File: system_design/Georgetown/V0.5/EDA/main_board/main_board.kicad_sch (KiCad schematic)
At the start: 23 parts, among them U1 top_rail_v2, U2 DS3231M, U3 INA219AxD, U5 KA78M05_TO252

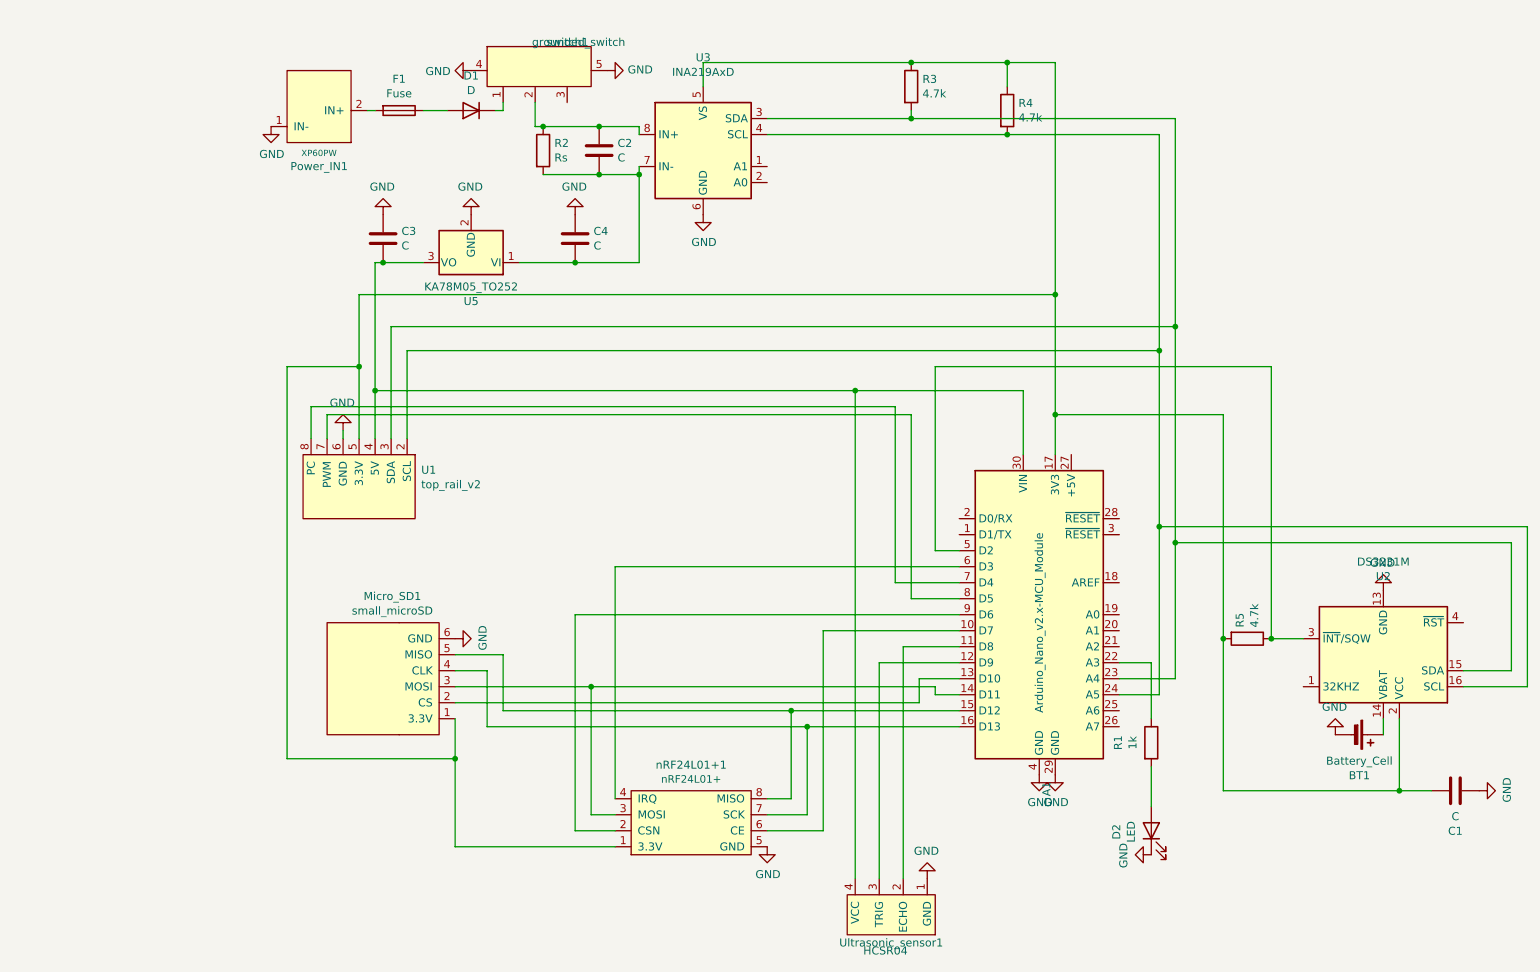
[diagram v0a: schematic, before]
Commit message: PCB modified
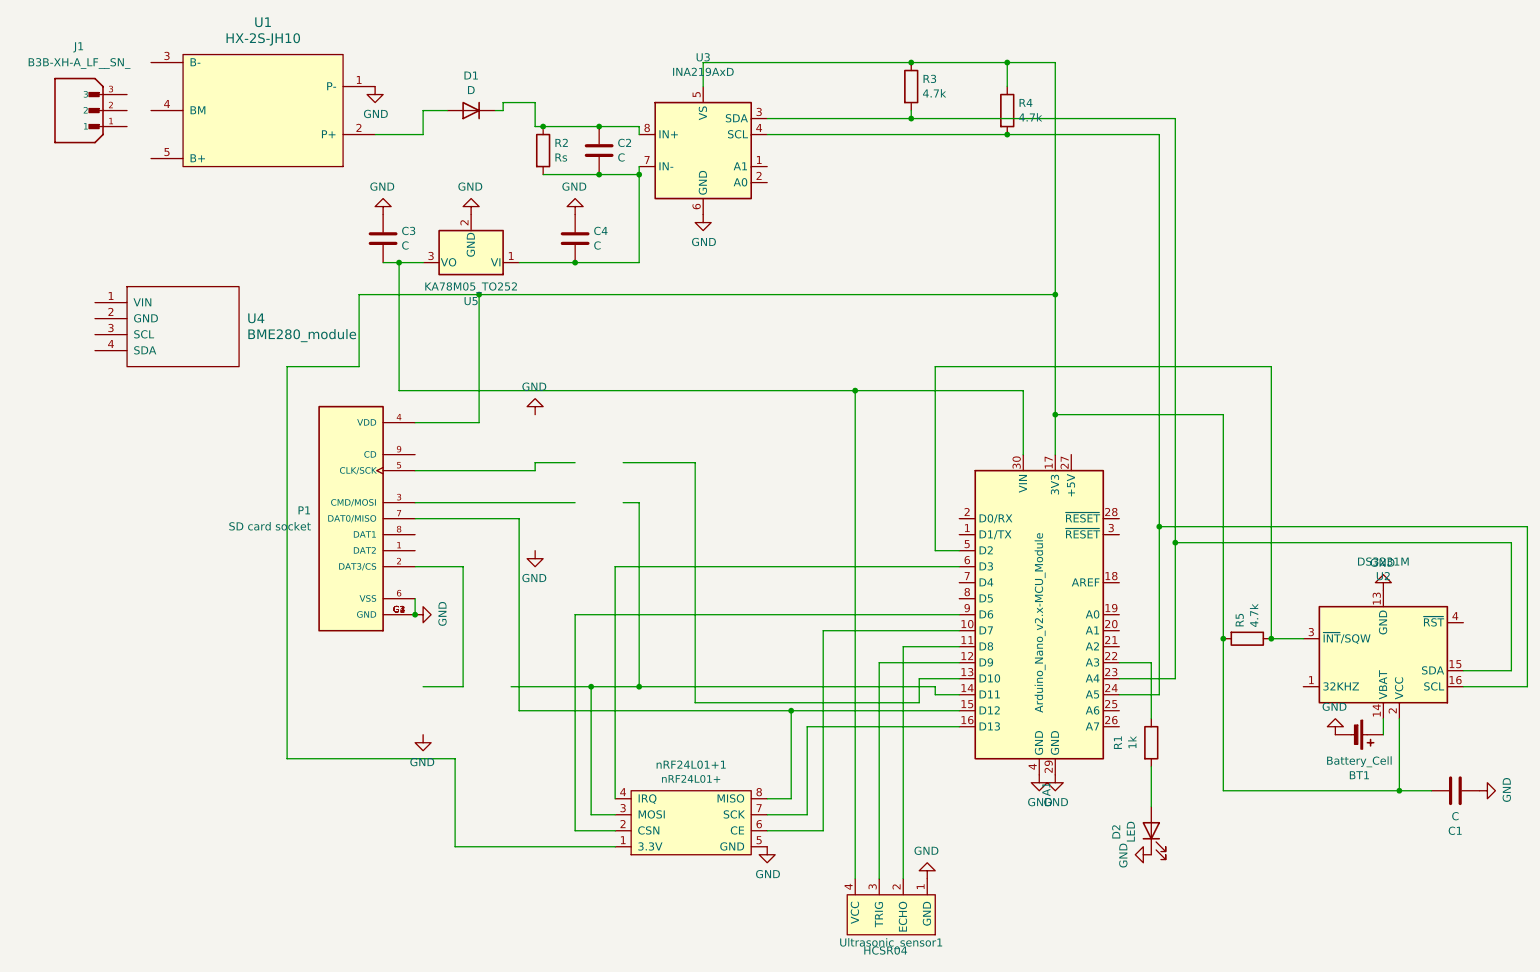
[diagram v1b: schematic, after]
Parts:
- removed F1: Fuse, Resistor_SMD:R_0603_1608Metric_Pad1.05x0.95mm_HandSolder, symbol Device:Fuse
- removed Micro_SD1: small_microSD, ARTS-Lab:small_microSD_v2, symbol main_board-rescue:small_microSD-whs5-rescue
- removed Power_IN1: XP60PW, ARTS-Lab:XT60PW, symbol main_board-rescue:XP60PW-whs5-rescue-whs5-rescue
- removed U1: top_rail_v2, ARTS-Lab:top_rail_v2, symbol main_board-rescue:top_rail_v2-ARTS-Lab
- removed switch1: grounded_switch, ARTS-Lab:grounded_switch, symbol main_board-rescue:grounded_switch-whs5-rescue-whs5-rescue
- added J1: B3B-XH-A_LF__SN_, XH2.54:XH2.54, symbol XH2.54:B3B-XH-A_LF__SN_
- added P1: SD card socket, ST-TF-003A:SUNTECH_ST-TF-003A, symbol ST-TF-003A:ST-TF-003A
- added U1: HX-2S-JH10, megasaturnv_custom_components:HX-2S-JH10, symbol megasaturnv_custom_components:HX-2S-JH10
- added U4: BME280_module, megasaturnv_custom_components:BME280_module, symbol megasaturnv_custom_components:BME280_module
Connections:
- net GND: now also P1.6 (VSS), P1.G1 (GND), P1.G2 (GND), P1.G3 (GND), P1.G4 (GND), U1.1 (P-)
- net at A1.17 (3V3), C1.1, R3.1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: now also P1.4 (VDD)
- net at A1.15 (D12), nRF24L01+1.8 (MISO): now also P1.7 (DAT0/MISO)
- net at D1.1 (K): now also C2.1, R2.1, U3.8 (IN+)
- net at D1.2 (A): now also U1.2 (P+)
